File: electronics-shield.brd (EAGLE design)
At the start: 85 x 56 mm, 86 parts, among them IC1 TLE9201SG, IC2 TLE9201SG, IC3 TLE9201SG, IC4 TLE9201SG, IC5 LINEAR_MCP1703CB, J1 USB-MICRO-B, Q1 USER-SUBMITTED_MOSFET-PCHANNE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, Q2 ON-SEMICONDUCTOR---NTZD3154NT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, Q3 ON-SEMICONDUCTOR---NTZD3154NT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, U1 STM32F0XX8T, U2 EEPROM-I2C, X1 CONNECTOR_PHOENIX_3.81, X2 Listwa zaciskowa rozłączalna 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, Y1 8 MHz

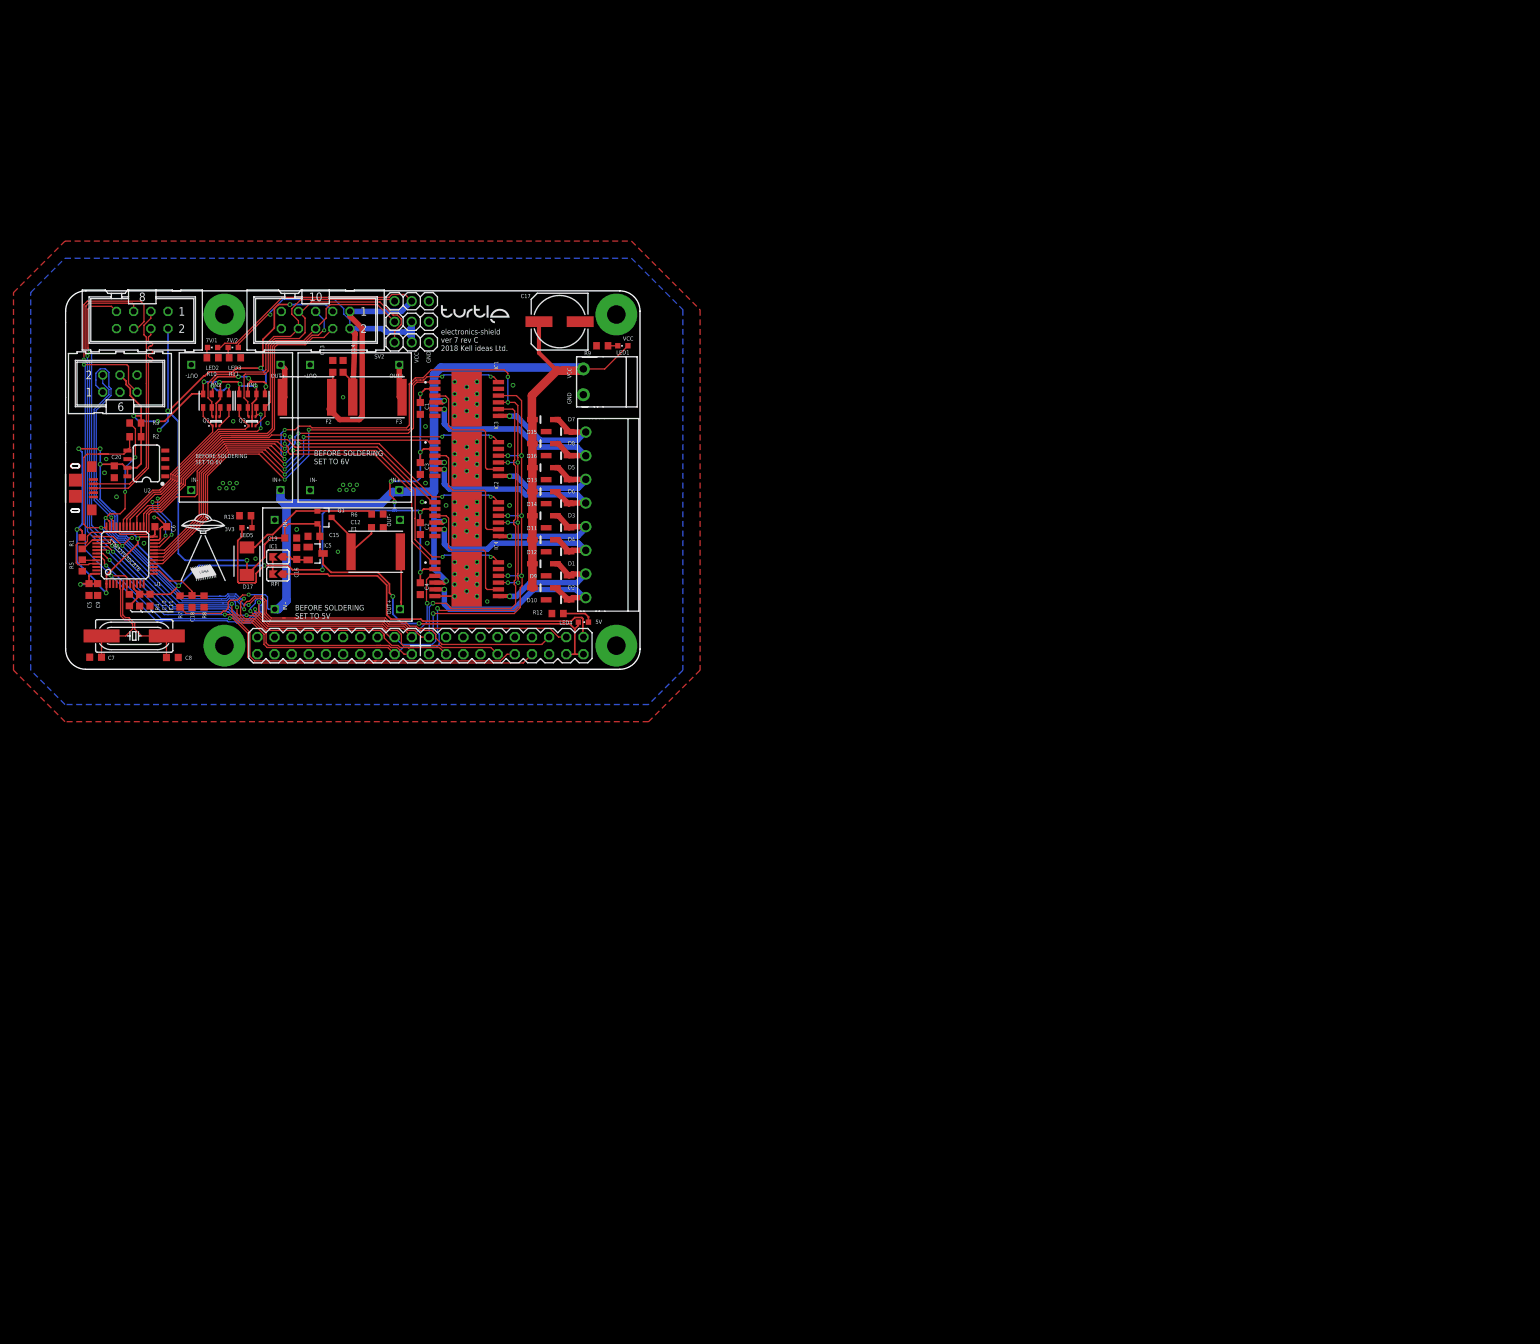
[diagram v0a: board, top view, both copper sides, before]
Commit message: Changed microprocessor, major and minor changes
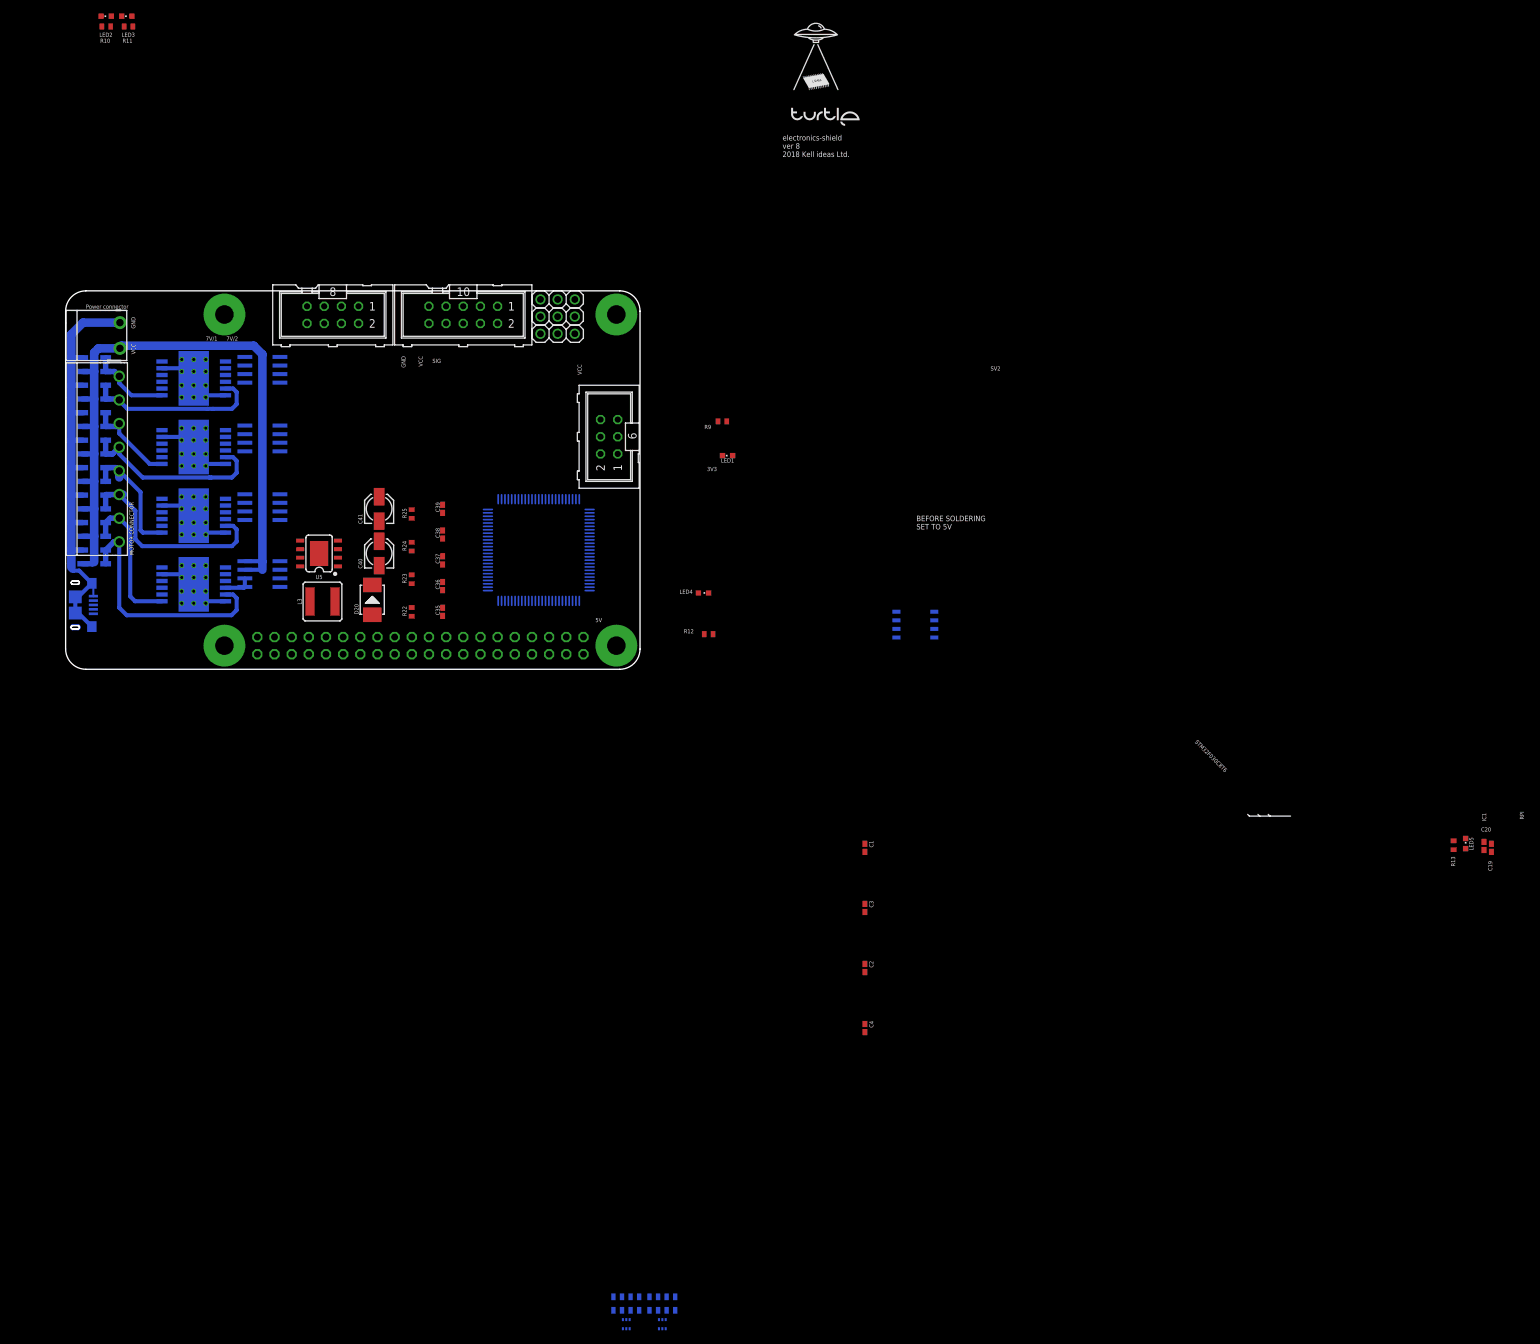
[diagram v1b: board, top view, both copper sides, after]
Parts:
- removed $3_0_$_2018-08-14_21-12-08, $3_1_$_2018-08-14_21-12-08, $3_2_$_2018-08-14_21-12-08: Moduł przetwornicy DC-DC Step-down 4.5..28V --- regulowane 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, Kell Ideas:DC-BRICK
- removed C10: 1u, Kell Ideas:C0603K
- removed C11, C12, C13, C14, C6, C9: 100n, Kell Ideas:C0603K
- removed C15: 4.7uF, Kell Ideas:C0603K
- removed C16: 1uF, Kell Ideas:C0603K
- removed C17: 100u, Kell Ideas:FI8_6.2
- removed C18: 22u, Kell Ideas:C0603K
- removed C5: 4u7, Kell Ideas:C0603K
- removed C7, C8: 20p, Kell Ideas:C0603K
- removed D17: SMBJ5.0A-TR, Kell Ideas:SMBJ
- removed F1, F2, F3: SL125-33, Kell Ideas:FUSC7351X125
- removed IC5: LINEAR_MCP1703CB, electronics-shield:LINEAR_SOT23
- removed Q1: USER-SUBMITTED_MOSFET-PCHANNELSMD, electronics-shield:USER-SUBMITTED_SOT23-3
- removed R1, R4, R5, R7: 10k, Kell Ideas:R0603
- removed R2, R3: 4k7, Kell Ideas:R0603
- removed R6: 100k, Kell Ideas:R0603
- removed R8: 1k, Kell Ideas:R0603
- removed SJ1, SJ2: (no value), Kell Ideas:SJ
- removed U1: STM32F0XX8T, Kell Ideas:LQFP48
- removed Y1: 8 MHz, Kell Ideas:HC49UP
- added C35, C36, C37, C38, C39: ?, Kell Ideas:C0402K
- added C40, C41: (no value), rcl:153CLV-0405
- added D20: 28V-5A, Seeed-Diode:DO-214AA
- added IC6, IC7, IC8, IC9: ACS712-LC, allegro-2:SOIC8
- added L3: ?, SparkFun-Coils:CR54
- added R22, R23, R24, R25: ?, Kell Ideas:R0402
- added U5: AOZ1284, Kell Ideas:SO-8_EXPOSED_PAD
- added U6: STM32F103VCT6, Kell Ideas:LQFP100
- C1, C19, C2, C20, C3, C4: device Kell Ideas:C0603K -> Kell Ideas:C0402K
- R10, R11, R12, R13, R9: device Kell Ideas:R0603 -> Kell Ideas:R0402
- moved C20 210.1 mm to (210.0, -26.0)
- moved LED5 186.3 mm to (207.3, -25.7), turned to 0 degrees
- moved R13 185.3 mm to (205.5, -25.9), turned to 270 degrees
- moved C19 183.5 mm to (211.1, -26.3), turned to 90 degrees
- moved Q2 146.7 mm to (83.1, -96.8), flipped to the bottom
- moved Q3 146.7 mm to (88.4, -96.8), flipped to the bottom
- moved RN1 146.7 mm to (88.4, -93.7), flipped to the bottom, turned to 180 degrees
- moved RN2 146.7 mm to (83.1, -93.7), flipped to the bottom, turned to 180 degrees
- moved U2 116.3 mm to (125.8, 6.74), flipped to the bottom, turned to 270 degrees
- moved C1 92.5 mm to (118.4, -26.3)
- moved C2 92.5 mm to (118.4, -44.1)
- moved C3 92.5 mm to (118.4, -35.2)
- moved C4 92.5 mm to (118.4, -53.0)
- moved D9 75.8 mm to (4.32, 46.2), flipped to the bottom, turned to 0 degrees
- moved D10 75.6 mm to (4.32, 42.2), flipped to the bottom, turned to 0 degrees
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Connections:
- removed net +5V_RAW: $3_0_$_2018-08-14_21-12-08.OUT1+1, F1.2
- removed net +7V/1_RAW: $3_1_$_2018-08-14_21-12-08.OUT1+1, F2.2
- removed net +7V/2_RAW: $3_2_$_2018-08-14_21-12-08.OUT1+1, F3.1
- removed net 3V3_STABILIZED: C16.1, IC5.2, SJ1.2
- removed net 5V_NOT_TRIMMED: C12.1, F1.1, Q1.3
- removed net BAT_MEAS: C18.1, R7.1, R8.2, U1.14
- removed net D1-R3: D17.A, Q1.1, R6.2
- removed net LED: U1.15
- removed net OSCILATOR_N: C7.2, U1.5, Y1.2
- removed net OSCILATOR_P: C8.2, U1.6, Y1.1
- removed net SEN1: U1.10
- removed net SEN2: U1.11
- removed net SEN3: U1.12
- removed net SEN4: U1.13
- new net BS2: C38.1, U5.2
- new net COMP: C37.1, U5.5
- new net C_COMP_R_COMP: C37.2, R25.2
- new net FB: R23.1, R24.2, U5.6
- new net FSW1: R22.2, U5.4
- new net LX: C38.2, D20.-, L3.P$1, U5.1
- new net N$10: U6.100, U6.11, U6.22, U6.28, U6.50, U6.75
- new net N$7: IC1.4, IC6.1, IC6.2
- new net N$9: U6.10, U6.19, U6.20, U6.27, U6.49, U6.74, U6.99
- new net NC: U6.73
- new net OSC_IN: U6.12
- new net OSC_OUT: U6.13
- new net PA0-WKUP: U6.23
- new net PA1: U6.24
- new net PA10: U6.69
- new net PA11: U6.70
- new net PA12: U6.71
- new net PA13: U6.72
- new net PA14: U6.76
- new net PA15: U6.77
- new net PA2: U6.25
- new net PA3: U6.26
- new net PA4: U6.29
- new net PA5: U6.30
- new net PA6: U6.31
- new net PA7: U6.32
- new net PA8: U6.67
- new net PA9: U6.68
- new net PB0: U6.35
- new net PB1: U6.36
- new net PB10: U6.47
- new net PB11: U6.48
- new net PB12: U6.51
- new net PB13: U6.52
- new net PB14: U6.53
- new net PB15: U6.54
- new net PB2: U6.37
- new net PB3: U6.89
- new net PB4: U6.90
- new net PB5: U6.91
- new net PB6: U6.92
- new net PB7: U6.93
- new net PB8: U6.95
- new net PB9: U6.96
- new net PC0: U6.15
- new net PC1: U6.16
- new net PC10: U6.78
- new net PC11: U6.79
- new net PC12: U6.80
- new net PC13-TAMPER-RTC: U6.7
- new net PC14-OSC32_IN: U6.8
- new net PC15-OSC32_OUT: U6.9
- new net PC2: U6.17
- new net PC3: U6.18
- new net PC4: U6.33
- new net PC5: U6.34
- new net PC6: U6.63
- new net PC7: U6.64
- new net PC8: U6.65
- new net PC9: U6.66
- new net PD0: U6.81
- new net PD1: U6.82
- new net PD10: U6.57
- new net PD11: U6.58
- new net PD12: U6.59
- new net PD13: U6.60
- new net PD14: U6.61
- new net PD15: U6.62
- new net PD2: U6.83
- new net PD3: U6.84
- new net PD4: U6.85
- new net PD5: U6.86
- new net PD6: U6.87
- new net PD7: U6.88
- new net PD8: U6.55
- new net PD9: U6.56
- new net PE0: U6.97
- new net PE1: U6.98
- new net PE10: U6.41
- new net PE11: U6.42
- new net PE12: U6.43
- new net PE13: U6.44
- new net PE14: U6.45
- new net PE15: U6.46
- new net PE2: U6.1
- new net PE3: U6.2
- new net PE4: U6.3
- new net PE5: U6.4
- new net PE6: U6.5
- new net PE7: U6.38
- new net PE8: U6.39
- new net PE9: U6.40
- new net SS1: C39.2, U5.7
- new net VBAT: U6.6
- new net VREF+: U6.21
- net +3V3: no longer C10.1, C11.1, C5.1, C6.1, C9.1, R1.2, R2.2, R3.2, R4.2, SJ1.1, SJ2.1, U1.1, U1.24, U1.48, U1.9
- net +5V: now also C35.1, C40.+, L3.P$2, R23.2; no longer C15.1, D17.C, IC5.3, Q1.2
- net +7V/1: no longer C13.1, F2.1
- net +7V/2: no longer C14.1, F3.2
- net 3V3_RPI: no longer SJ2.2
- net BOOT0: now also U6.94; no longer R5.2, U1.44
- net EN1: no longer U1.16
- net EN2: no longer U1.17
- net EN3: no longer U1.18
- net EN4: no longer U1.19
- net GND: now also C35.2, C36.2, C39.1, C40.-, C41.-, D20.+, IC6.5, IC7.5, IC8.5, IC9.5, R22.1, R24.1, R25.1, U5.3; no longer $3_0_$_2018-08-14_21-12-08.IN1-1, $3_0_$_2018-08-14_21-12-08.OUT1-1, $3_1_$_2018-08-14_21-12-08.IN1-1, $3_1_$_2018-08-14_21-12-08.OUT1-1, $3_2_$_2018-08-14_21-12-08.IN1-1, $3_2_$_2018-08-14_21-12-08.OUT1-1, C10.2, C11.2, C12.2, C13.2, C14.2, C15.2, C16.2, C17.-, C18.2, C5.2, C6.2, C7.1, C8.1, C9.2, IC5.1, R5.1, R6.1, R8.1, U1.23, U1.47, U1.8
- net IN11: no longer U1.45
- net IN21: no longer U1.32
- net IN31: no longer U1.25
- net IN41: no longer U1.27
- net MOT11: now also X2.8; no longer X2.7
- net MOT12: now also X2.7; no longer X2.8
- net MOT21: now also X2.6; no longer X2.5
- net MOT22: now also X2.5; no longer X2.6
- net MOT31: now also X2.4; no longer X2.3
- net MOT32: now also X2.3; no longer X2.4
- net MOT41: now also X2.2; no longer X2.1
- net MOT42: now also X2.1; no longer X2.2
- net NRST: now also U6.14; no longer R4.1, U1.7
- net RPI_CLK: no longer U1.39
- net RPI_MISO: no longer U1.40
- net RPI_MOSI: no longer U1.41
- net RPI_RXD: no longer U1.42
- net RPI_TXD: no longer U1.43
- net SCL: no longer R3.1, U1.35
- net SCL_TX: no longer U1.21
- net SDA: no longer R2.1, U1.36
- net SDA_RX: no longer U1.22
- net SERVO1_UC: no longer U1.29
- net SERVO2_UC: no longer U1.30
- net SERVO3_UC: no longer U1.31
- net SPI1_NSS: no longer R1.1, U1.38
- net SWCLK: no longer U1.37
- net SWDIO: no longer U1.34
- net TLE_NSS: no longer U1.20
- net VCC: now also C36.1, C41.+, IC6.3, IC6.4, IC6.8, IC7.8, IC8.8, IC9.8, U5.P$1; no longer $3_0_$_2018-08-14_21-12-08.IN1+1, $3_1_$_2018-08-14_21-12-08.IN1+1, $3_2_$_2018-08-14_21-12-08.IN1+1, C17.+, IC1.4, R7.2
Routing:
- net +3V3: track 258.0 -> 0.00 mm, vias 22 -> 0
- net +5V: track 180.3 -> 0.00 mm, vias 12 -> 0
- net RPI_MOSI: track 160.1 -> 0.00 mm, vias 4 -> 0
- net RPI_CLK: track 160.1 -> 0.00 mm, vias 10 -> 0
- net NRST: track 120.0 -> 0.00 mm, vias 3 -> 0
- net TLE_NSS: track 118.1 -> 0.00 mm, vias 10 -> 0
- net RPI_MISO: track 111.1 -> 0.00 mm, vias 4 -> 0
- net SDA: track 104.0 -> 0.00 mm, vias 2 -> 0
- net GND: track 9.94 -> 108.9 mm, vias 77 -> 48
- net SCL: track 97.9 -> 0.00 mm, vias 4 -> 0
- net SWCLK: track 93.1 -> 0.00 mm, vias 3 -> 0
- net VCC: track 199.9 -> 107.6 mm, vias 5 -> 0
- net SWDIO: track 88.0 -> 0.00 mm, vias 2 -> 0
- net SPI1_NSS: track 80.4 -> 0.00 mm, vias 3 -> 0
- net IN11: track 78.6 -> 0.00 mm, vias 2 -> 0
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- removed copper zone on layer 1, net GND
- removed copper zone on layer 16, net GND
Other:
- board text added: "electronics-shield ver 8 2018 Kell ideas Ltd."
- board text removed: "BEFORE SOLDERING SET TO 6V"
- board text removed: "electronics-shield ver 7 rev C 2018 Kell ideas Ltd."
